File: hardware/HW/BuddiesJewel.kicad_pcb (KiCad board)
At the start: 2 copper layers, 22 parts, among them CON1 AVR-ISP6, CON2 ANTENNE, IC1 ATTINY25-P, P1 ALIM, U1 PT, U2 PT, U3 PT, U4 PT, U5 RF430CL330H

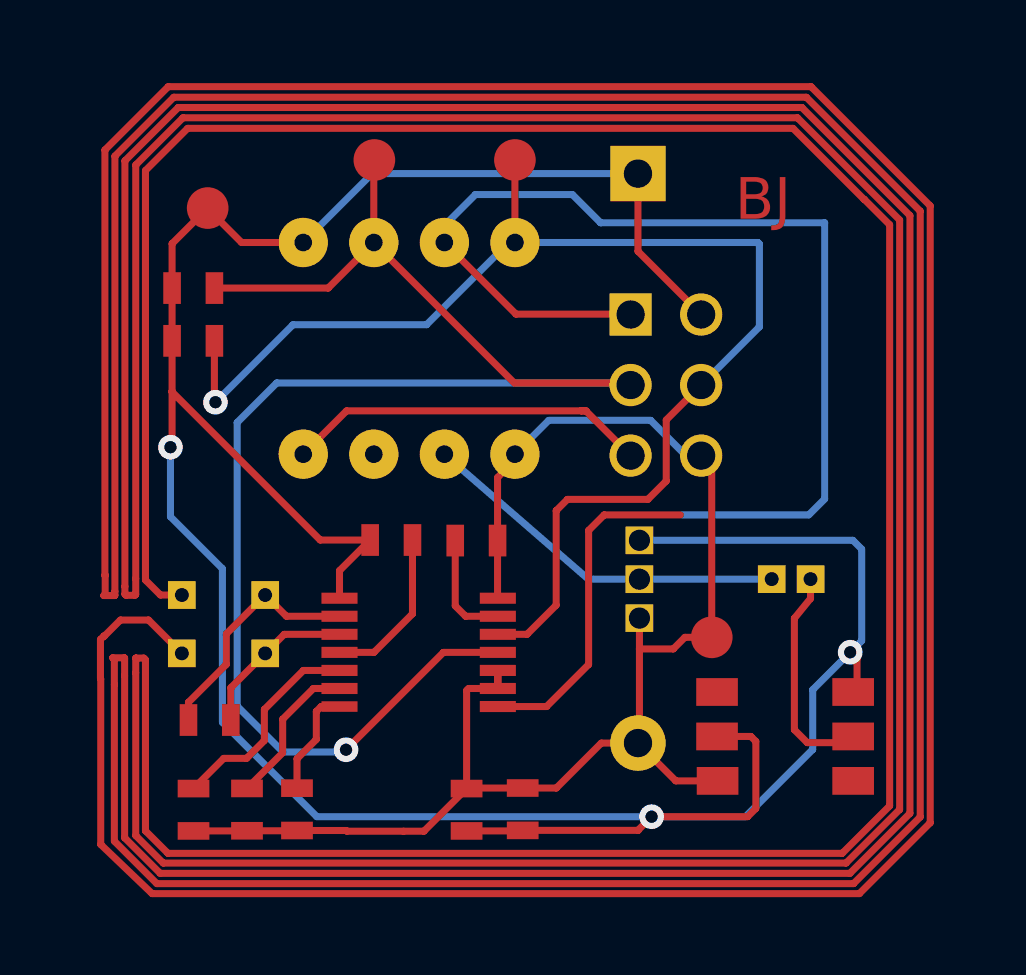
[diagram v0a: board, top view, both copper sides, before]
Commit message: new antenna and some enhanced stuff
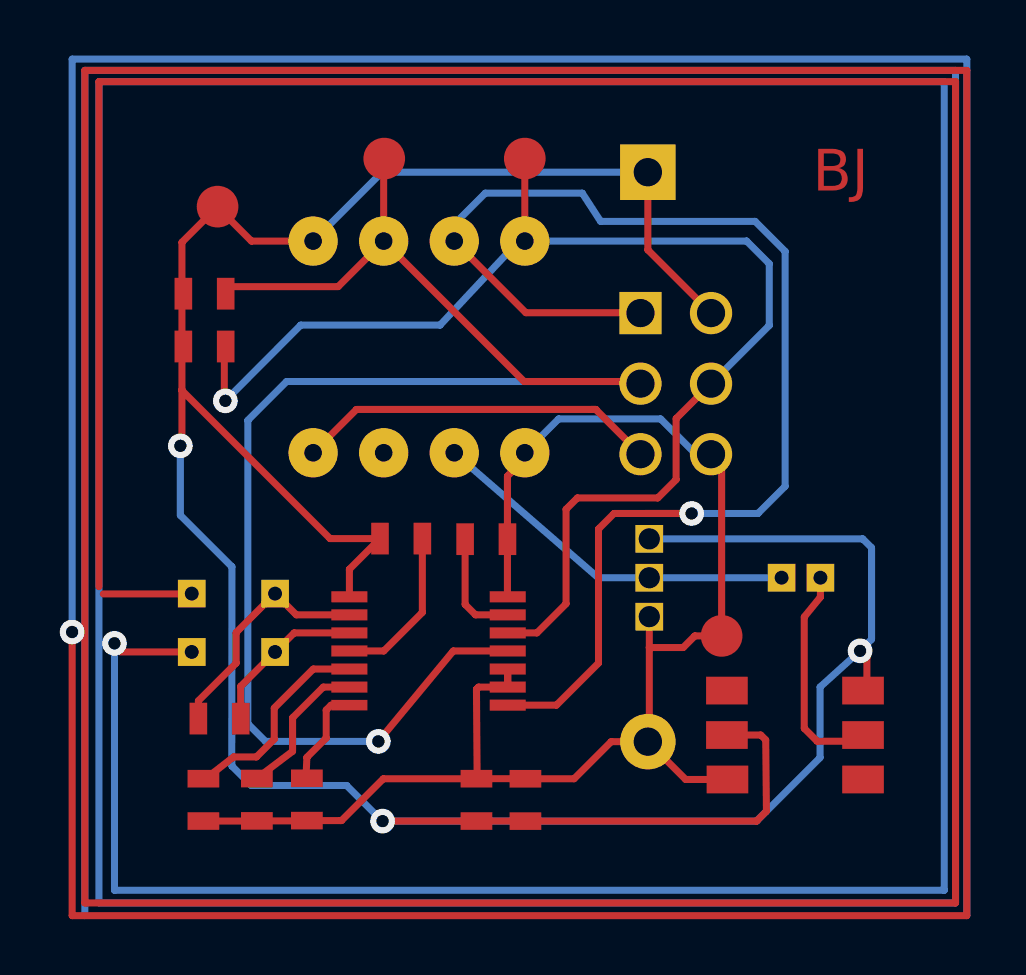
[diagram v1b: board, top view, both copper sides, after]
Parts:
- moved R5 0.50 mm to (56.8, 52.5)
- moved R6 0.50 mm to (58.6, 52.5)
- moved C1 0.50 mm to (64.7, 52.5)
- moved R4 0.50 mm to (54.9, 52.5)
- moved R2 0.45 mm to (55.0, 36.2)
- moved R1 0.45 mm to (55.0, 34.3)
- moved D2 0.36 mm to (71.0, 43.1)
- moved U4 0.36 mm to (66.5, 29.4)
- moved CON1 0.36 mm to (71.9, 37.5)
- moved IC1 0.36 mm to (62.7, 36.2)
- moved R3 0.36 mm to (62.0, 43.1)
- moved U5 0.36 mm to (60.2, 45.2)
- moved U1 0.36 mm to (61.4, 29.4)
- moved U2 0.36 mm to (55.4, 31.2)
- moved C4 0.36 mm to (55.5, 49.6)
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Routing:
- net (no net): track 0.00 -> 328.2 mm, vias 0 -> 1
- net N-0000012: track 527.1 -> 256.2 mm, vias 0 -> 1
- net +3.3V: track 110.9 -> 115.6 mm
- net /IT/MISO: track 50.5 -> 47.9 mm, vias 0 -> 1

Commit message: new PCB revision
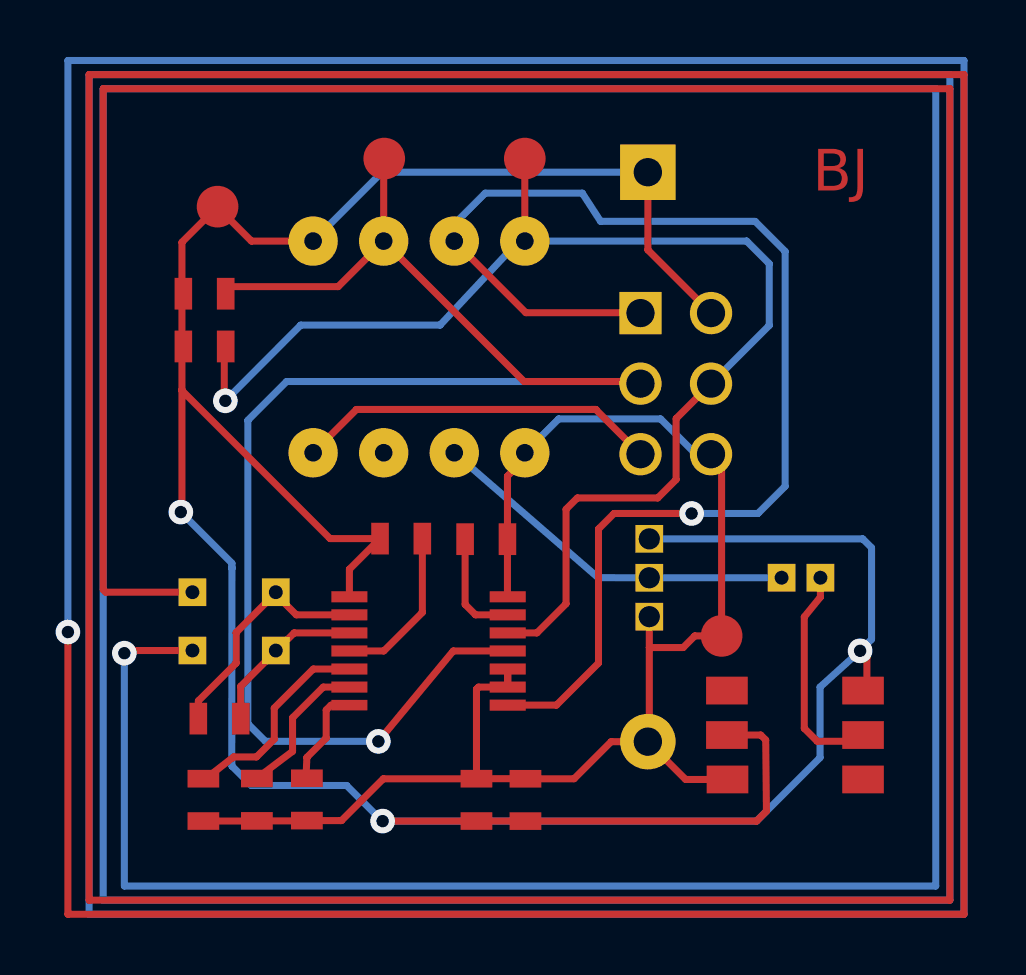
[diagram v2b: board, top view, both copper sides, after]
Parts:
- moved CON2 0.06 mm to (57.5, 45.0)
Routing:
- net N-0000012: track 256.2 -> 610.0 mm, vias 1 -> 2
- net (no net): track 328.2 -> 0.00 mm, vias 1 -> 0
